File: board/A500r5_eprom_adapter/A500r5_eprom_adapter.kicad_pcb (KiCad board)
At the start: 2 copper layers, 45.7 x 86.4 mm, 10 parts, among them J1 PWR, J2 A18 Selector, J3 A19 Selector, U1 27C400-A500, U2 27C080-L, U3 27C080-L

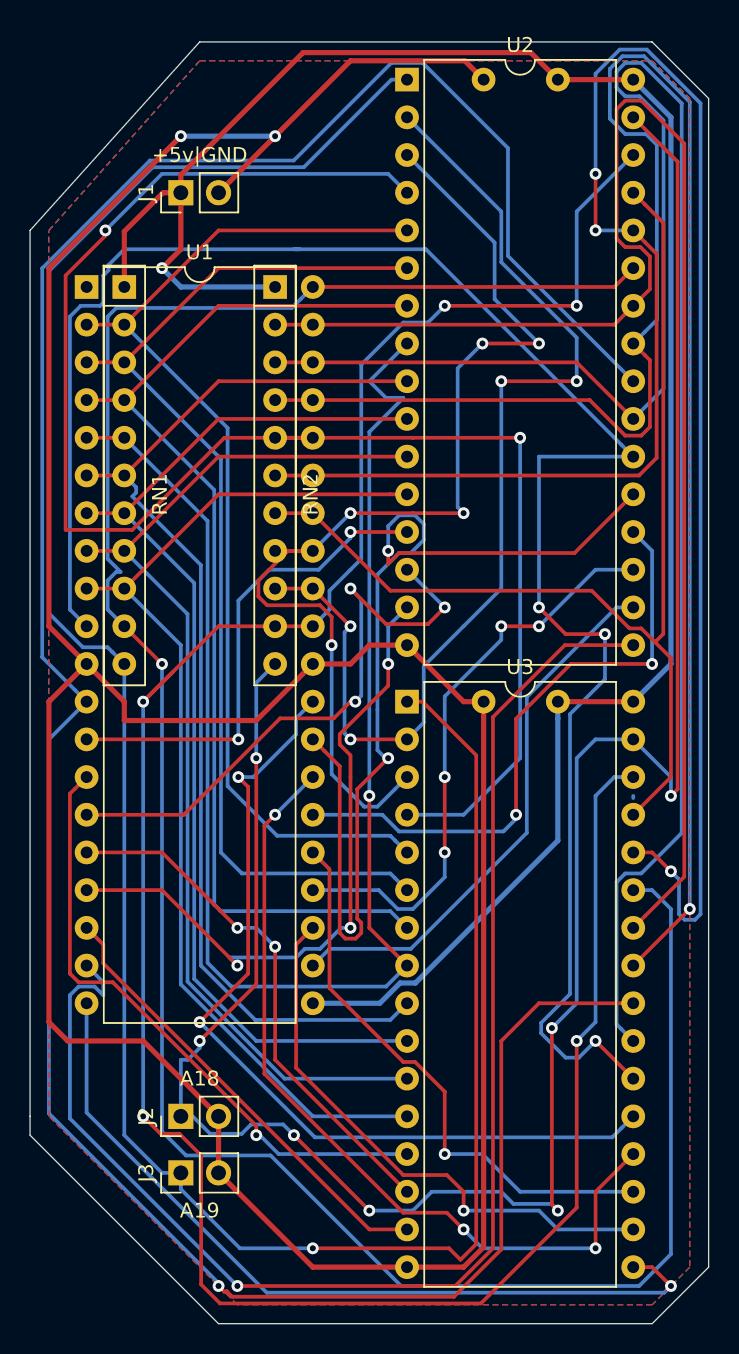
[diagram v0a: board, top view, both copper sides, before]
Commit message: add rev 1 for DIP adapter
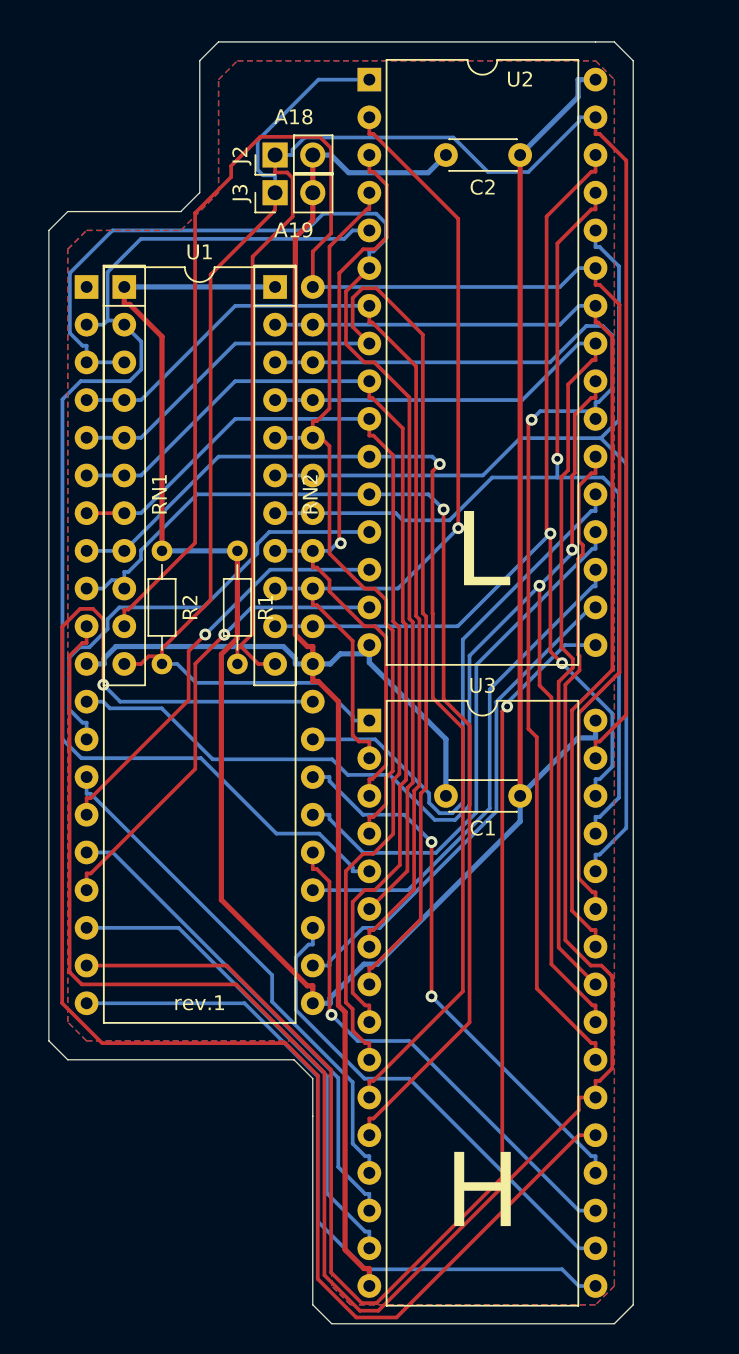
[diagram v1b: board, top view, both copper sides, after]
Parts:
- removed J1: PWR, Connector_PinHeader_2.54mm:PinHeader_1x02_P2.54mm_Vertical
- added R1: 4k7, Resistor_THT:R_Axial_DIN0204_L3.6mm_D1.6mm_P7.62mm_Horizontal, F.Cu at (116.8, 88.9)
- added R2: 4k7, Resistor_THT:R_Axial_DIN0204_L3.6mm_D1.6mm_P7.62mm_Horizontal, F.Cu at (111.8, 88.9)
- C1, C2: moved to F.Cu
- moved J3 66.3 mm to (119.4, 64.8)
- moved J2 65.1 mm to (119.4, 62.2)
- moved C1 6.84 mm to (135.9, 105.4)
- moved C2 5.68 mm to (135.9, 62.2)
- moved U3 2.84 mm to (125.7, 100.3)
- moved U2 2.54 mm to (125.7, 57.1)
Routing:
- net /A17: track 164.7 -> 68.3 mm, vias 5 -> 2
- net /A19: track 158.1 -> 67.1 mm, vias 1 -> 0
- net /~OE: track 179.0 -> 92.8 mm, vias 1 -> 2
- net GND: track 202.3 -> 122.4 mm, vias 2 -> 0
- net /A12: track 110.2 -> 51.6 mm, vias 2 -> 0
- net /A13: track 127.1 -> 69.2 mm, vias 3 -> 0
- net /A11: track 120.6 -> 69.2 mm, vias 1 -> 0
- net /D7-H: track 58.9 -> 105.8 mm, vias 2 -> 1
- net /A10: track 123.7 -> 80.0 mm, vias 0 -> 1
- net /A8: track 159.9 -> 117.2 mm, vias 1 -> 0
- net /A18: track 151.8 -> 109.8 mm, vias 7 -> 0
- net /D7-L: track 70.2 -> 37.5 mm, vias 2 -> 0
- net /A9: track 100.2 -> 67.8 mm
- net /A4: track 101.5 -> 77.1 mm, vias 1 -> 0
- net /A15: track 74.7 -> 53.0 mm, vias 5 -> 1
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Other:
- board size 45.7 x 86.4 mm -> 39.4 x 86.4 mm
- board text added: "H"
- board text added: "L"
- board text added: "rev.1"
- board text removed: "+5v|GND"
